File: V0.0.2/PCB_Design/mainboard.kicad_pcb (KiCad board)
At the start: 2 copper layers, 48.3 x 58.4 mm, 11 parts, among them U1 DS3231M, U2 CR1025, U3 Rails, U4 MicroSD.V2, U5 Battery, U6 Phsensor

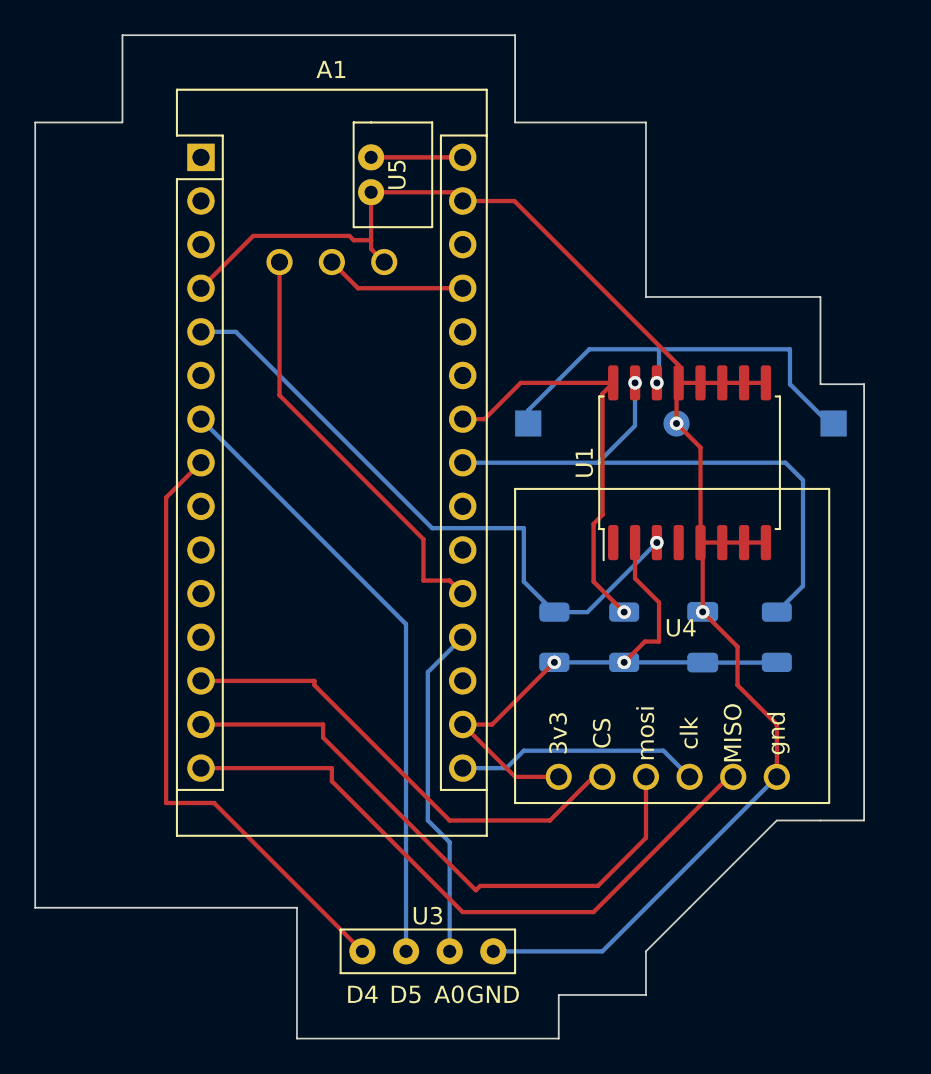
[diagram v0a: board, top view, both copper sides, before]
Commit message: Gibson, Daniel
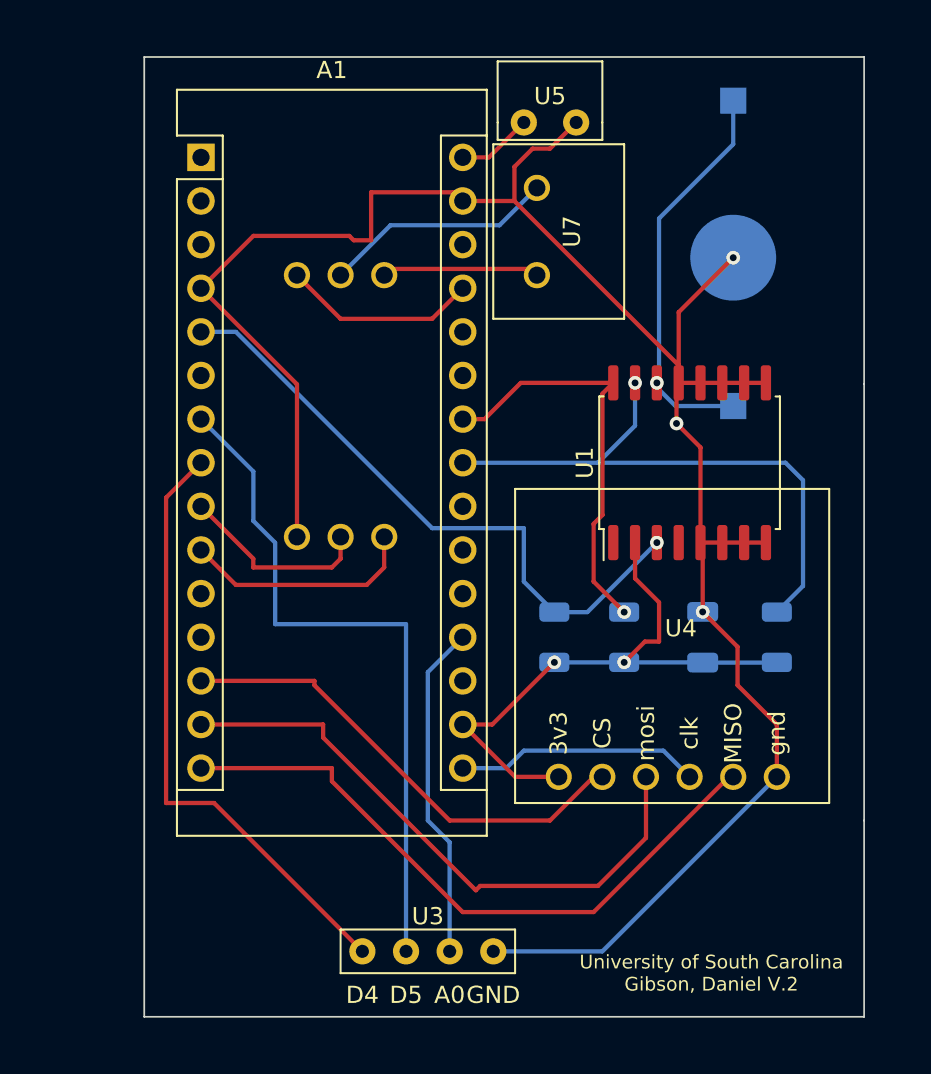
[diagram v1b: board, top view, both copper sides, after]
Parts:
- added U7: Probe_slot, Water_sensor:Probe_rails, F.Cu at (113.0, 62.2)
- R4: value R -> 4.7K
- U6: value Phsensor -> Ph_embedded; footprint Water_sensor:PH_meter -> Water_sensor:pH_embedded
- moved U2 16.6 mm to (121.9, 57.1), turned to 0 degrees
- moved U5 9.80 mm to (111.3, 53.8), turned to 0 degrees
- moved U6 4.35 mm to (99.1, 67.3)
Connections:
- U6 pad 1: Net-(A1-Pad20) -> GND
- U6 pad 2: Net-(A1-Pad27) -> Net-(A1-Pad9)
- U6 pad 3: GND -> Net-(A1-Pad10)
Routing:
- net GND: track 93.8 -> 124.2 mm, vias 2 -> 3
- net Net-(A1-Pad20): track 24.6 -> 0.00 mm
- net Net-(A1-Pad10): track 0.00 -> 13.7 mm
- net Net-(U6-Pad5): track 0.00 -> 13.5 mm
- net Net-(A1-Pad9): track 0.00 -> 11.4 mm
- net Net-(U6-Pad6): track 0.00 -> 9.19 mm
- net Net-(A1-Pad7): track 35.9 -> 40.4 mm
- net Net-(A1-Pad27): track 8.25 -> 11.4 mm
- net Net-(U1-Pad14): track 25.0 -> 23.4 mm
- net Net-(A1-Pad30): track 5.33 -> 4.40 mm
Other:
- board size 48.3 x 58.4 mm -> 41.9 x 55.9 mm
- board text added: "University of South Carolina Gibson, Daniel V.2"
